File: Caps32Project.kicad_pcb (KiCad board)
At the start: 2 copper layers, 20 x 33 mm, 23 parts, among them J1 Ph 2.0, J2 Sh 1.0, P1 USB_C_Plug_USB2.0, Q1 AO3401A, U1 MPU-6050, U2 MAX17048G_T10, U3 ESP32C3_SuperMini, U4 MCP73831-2-OT

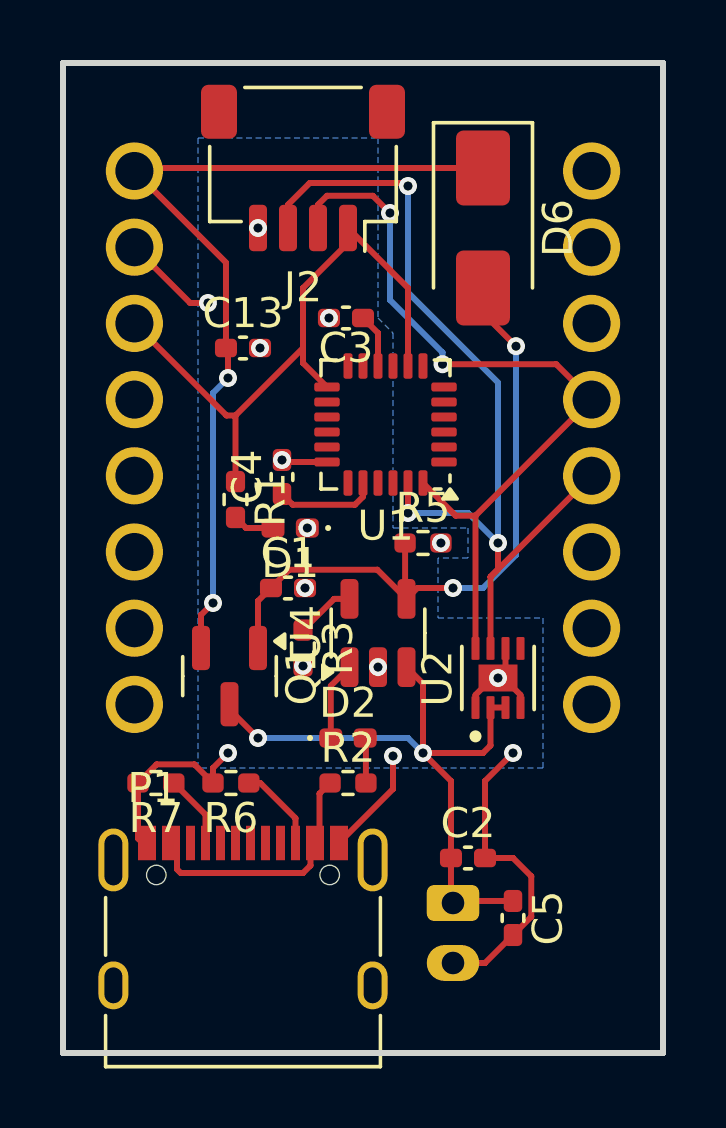
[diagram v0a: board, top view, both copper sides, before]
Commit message: LGTM
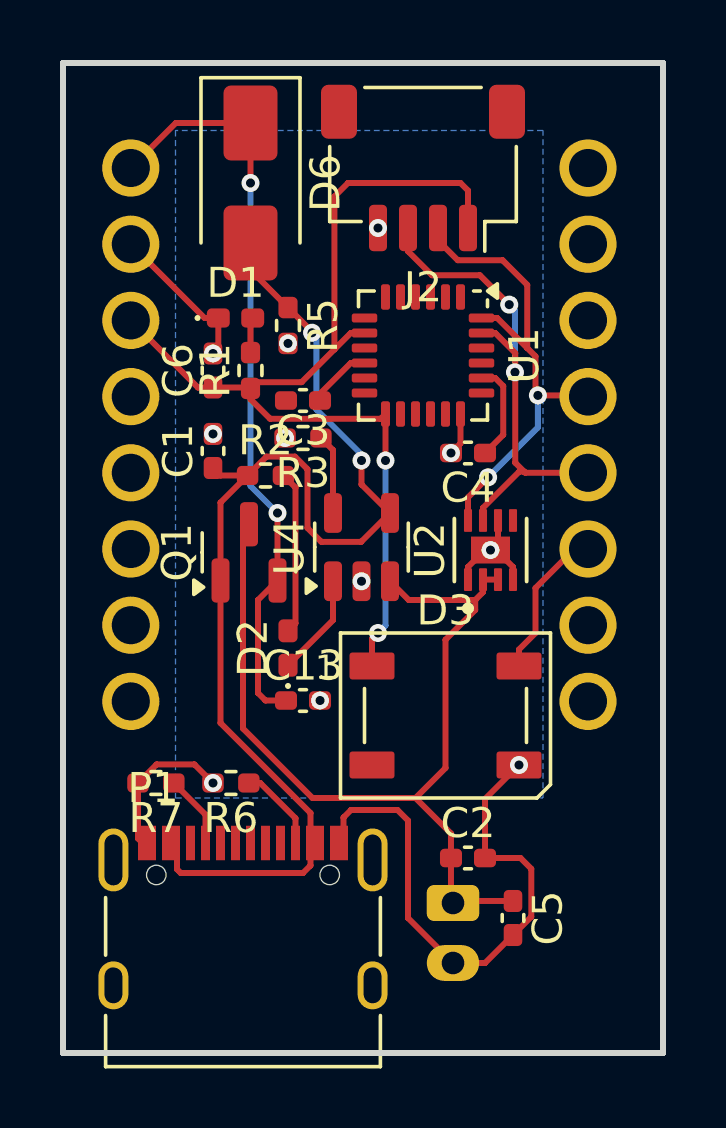
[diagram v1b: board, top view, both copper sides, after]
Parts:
- added C6: 1.0uF, Capacitor_SMD:C_0402_1005Metric_Pad0.74x0.62mm_HandSolder, F.Cu at (187.0, 56.8)
- added D3: WS2812B, LED_SMD:LED_WS2812B_PLCC4_5.0x5.0mm_P3.2mm, F.Cu at (194.8, 68.2)
- moved C13 11.9 mm to (190.0, 67.8)
- moved R2 10.6 mm to (188.8, 60.2)
- moved R5 8.53 mm to (189.5, 55.2), turned to -90 degrees
- moved D6 7.89 mm to (188.2, 50.5)
- moved D1 7.23 mm to (187.8, 55.0), turned to 0 degrees
- moved R3 7.00 mm to (190.0, 59.0), turned to 180 degrees
- moved C4 6.25 mm to (195.5, 59.5), turned to 180 degrees
- moved C1 5.21 mm to (187.0, 59.4), turned to 90 degrees
- moved R1 4.33 mm to (188.2, 56.8), turned to 90 degrees
- moved U2 4.27 mm to (196.2, 62.7)
- moved Q1 4.18 mm to (188.2, 62.8), turned to 90 degrees
- moved J2 4.00 mm to (194.0, 50.0)
- moved D2 3.61 mm to (189.5, 66.0), turned to 90 degrees
- moved C3 3.10 mm to (190.0, 57.8)
- moved U4 2.91 mm to (191.9, 62.6)
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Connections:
- U3 pad 10: unconnected-(U3-GPIO10-Pad10) -> RGB
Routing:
- net SCL: track 31.1 -> 17.2 mm, vias 3 -> 2
- net +3V3: track 21.7 -> 34.3 mm, vias 0 -> 2
- net SDA: track 26.9 -> 16.6 mm
- net +BATT: track 21.9 -> 31.5 mm, vias 2 -> 0
- net VBUS: track 31.4 -> 40.2 mm
- net RGB: track 0.00 -> 6.92 mm
- net GND: track 29.0 -> 34.3 mm, vias 14 -> 11
- net Net-(D2-A): track 1.51 -> 5.45 mm
- net +5V: track 29.2 -> 25.3 mm
- net Net-(D2-K): track 2.62 -> 3.42 mm
- net Net-(U4-PROG): track 1.98 -> 2.67 mm
